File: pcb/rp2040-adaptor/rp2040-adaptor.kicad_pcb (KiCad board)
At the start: 2 copper layers, 35 x 29 mm, 3 parts, among them J1 Conn_01x09, J2 Conn_01x09

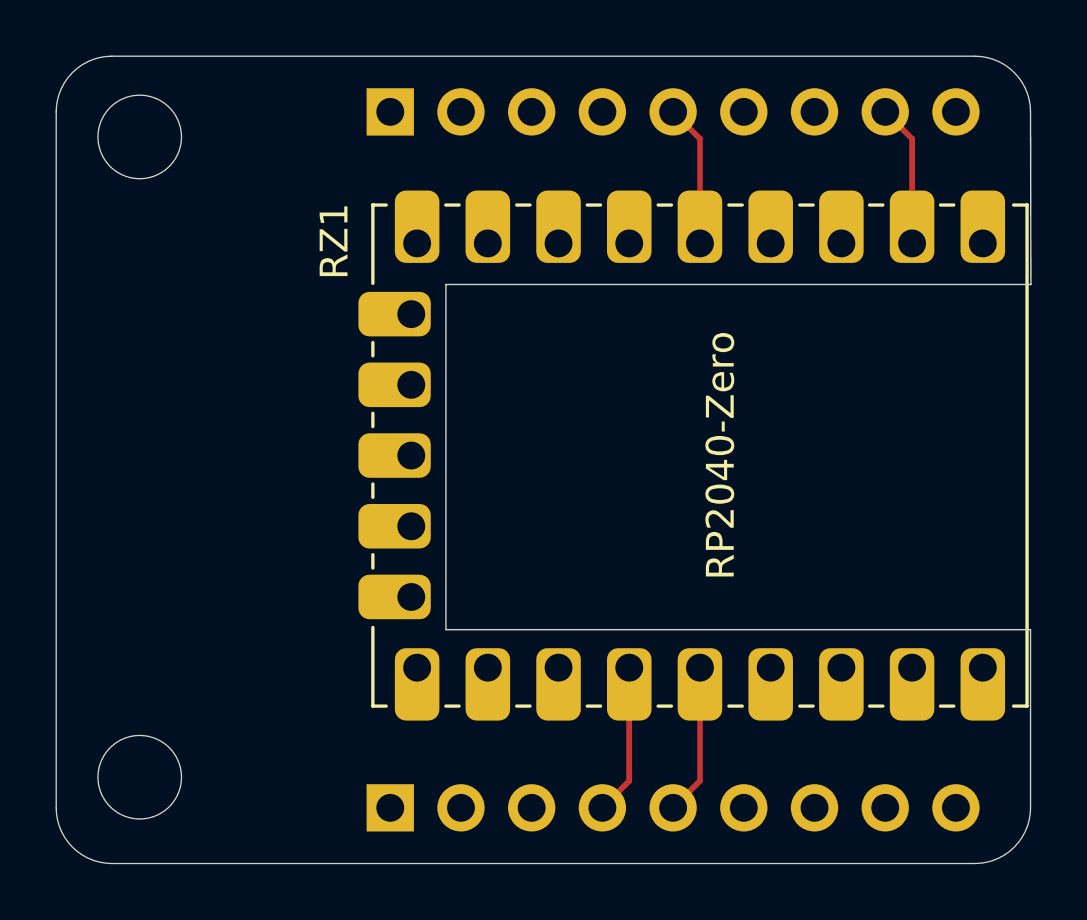
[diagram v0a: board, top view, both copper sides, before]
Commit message: correct hardware bugs
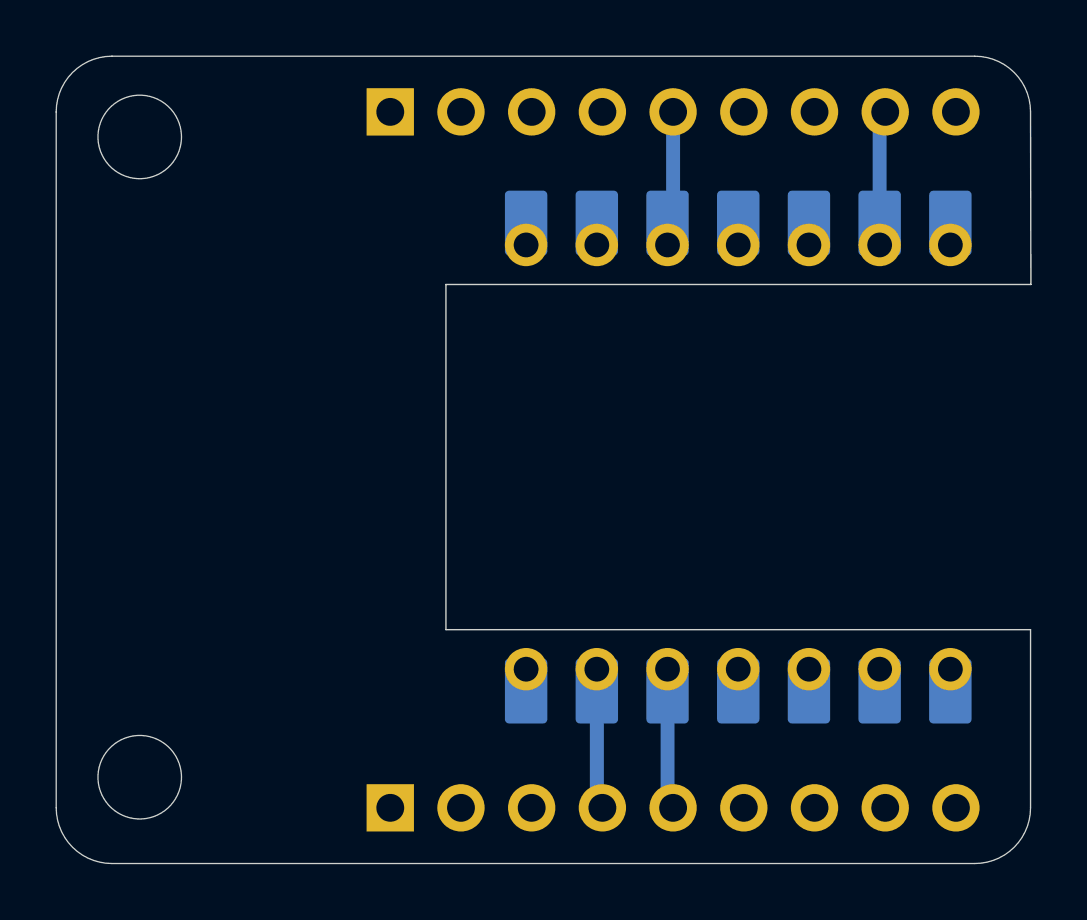
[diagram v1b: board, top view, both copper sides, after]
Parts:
- RZ1: value RP2040-Zero -> XIAO-RP2350; footprint library:RP2040-Zero -> library:XIAO-RP2350-DIP; moved to B.Cu
- moved RZ1 17.4 mm to (119.0, 86.8), turned to 0 degrees
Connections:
- RZ1 pad 10: unconnected-(RZ1-GP9-Pad10) -> CEC
- RZ1 pad 13: unconnected-(RZ1-GP12-Pad13) -> GND
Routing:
- net SDA: track 5.43 -> 4.28 mm
- net SCL: track 5.43 -> 4.28 mm
- net CEC: track 5.12 -> 4.08 mm
